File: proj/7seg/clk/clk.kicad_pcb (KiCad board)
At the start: 2 copper layers, 63.2 x 12.8 mm, 26 parts, among them J1 Conn_01x02_Pin, J2 Conn_01x04_Pin, SW1 SW_Push, SW2 SW_Push, U1 LTC-4627JG, U2 74HC595, U3 74HC595, U4 ATtiny402-SS

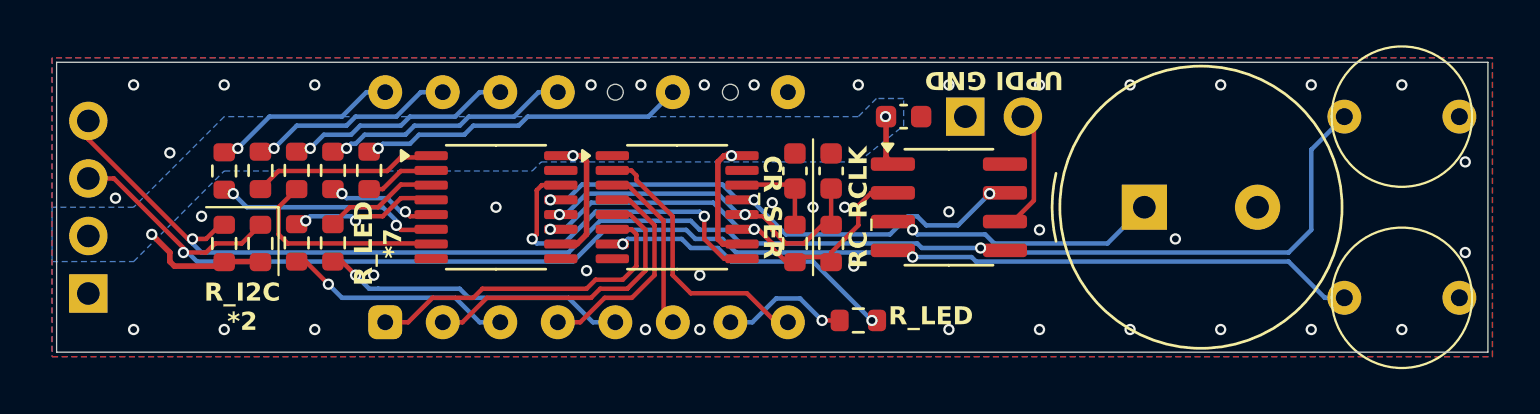
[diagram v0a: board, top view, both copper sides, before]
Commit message: -
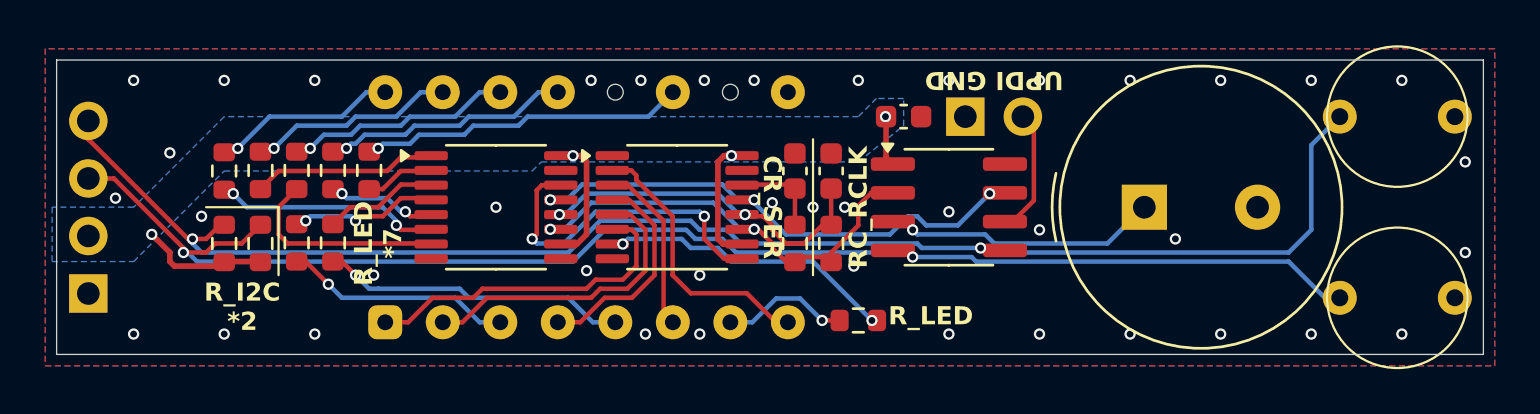
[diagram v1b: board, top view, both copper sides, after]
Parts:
- moved G*** 1.00 mm to (128.0, 97.0), turned to 180 degrees
- moved SW1 0.20 mm to (135.8, 104.0)
- moved SW2 0.20 mm to (135.8, 96.0)
- turned ? to 180 degrees
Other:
- board size 63.2 x 12.8 mm -> 63 x 13 mm
- board text added: "AVR_CLK"
